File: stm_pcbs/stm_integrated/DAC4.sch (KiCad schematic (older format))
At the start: 21 parts, among them P4 BNC, U10 AD8676, U11 AD5791, U12 AD8675

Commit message: working on Kicad of 3rd Dec
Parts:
- C49, C51, C53, C55, C56, C59, C60, C63, C64: symbol C -> device:C
- C50, C52, C54, C57, C58, C61, C62: symbol CP2 -> device:CP1
- P4: symbol BNC -> device:BNC
- R4: symbol R -> device:R
- U10: symbol AD8676 -> ad5791:AD8676
- U11: symbol AD5791 -> ad5791:AD5791
- U12: symbol AD8675 -> ad5791:AD8675
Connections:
- wire segments 111 -> 126
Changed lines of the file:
@@
-EESchema Schematic File Version 2
-LIBS:power
-LIBS:device
-LIBS:transistors
-LIBS:conn
-LIBS:linear
-LIBS:regul
-LIBS:74xx
-LIBS:cmos4000
-LIBS:adc-dac
-LIBS:memory
-LIBS:xilinx
-LIBS:special
-LIBS:microcontrollers
-LIBS:dsp
-LIBS:microchip
-LIBS:analog_switches
-LIBS:motorola
-LIBS:texas
-LIBS:intel
-LIBS:audio
-LIBS:interface
-LIBS:digital-audio
-LIBS:philips
-LIBS:display
-LIBS:cypress
-LIBS:siliconi
-LIBS:opto
-LIBS:atmel
-LIBS:contrib
-LIBS:valves
-LIBS:ad5791
+EESchema Schematic File Version 4
 LIBS:stmshieldfull-cache
-LIBS:powerbrd-cache
-LIBS:LTC1859-cache
-EELAYER 25 0
+EELAYER 26 0
 EELAYER END
 $Descr A4 11693 8268
@@
 $EndDescr
 $Comp
-L AD5791 U11
+L ad5791:AD5791 U11
 U 1 1 5A26063E
 P 5150 3800
@@
 $EndComp
 $Comp
-L AD8675 U12
+L ad5791:AD8675 U12
 U 1 1 5A260645
 P 6850 3450
@@
 $EndComp
 $Comp
-L AD8676 U10
+L ad5791:AD8676 U10
 U 1 1 5A26064C
 P 5050 1750
@@
 $EndComp
 $Comp
-L AD8676 U10
+L ad5791:AD8676 U10
 U 2 1 5A260653
 P 5100 5500
@@
 $EndComp
 $Comp
-L AD8676 U10
+L ad5791:AD8676 U10
 U 3 1 5A26065A
 P 7800 5600
@@
 $EndComp
 $Comp
-L BNC P4
+L device:BNC P4
 U 1 1 5A260661
 P 7950 3450
@@
 -14V
 $Comp
-L AGND #PWR037
+L power:AGND #PWR037
 U 1 1 5A26066E
 P 7950 3800
@@
 3.3V
 $Comp
-L AGND #PWR038
+L power:AGND #PWR038
 U 1 1 5A260677
 P 4950 4900
@@
 $EndComp
 $Comp
-L DGND #PWR039
+L power:DGND #PWR039
 U 1 1 5A26067D
 P 4700 4900
@@
 $EndComp
 $Comp
-L C C51
+L device:C C51
 U 1 1 5A260683
 P 5950 2200
@@
 $EndComp
 $Comp
-L AGND #PWR040
+L power:AGND #PWR040
 U 1 1 5A26068A
 P 6400 2350
@@
 $EndComp
 $Comp
-L C C53
+L device:C C53
 U 1 1 5A260690
 P 6100 4600
@@
 $EndComp
 $Comp
-L AGND #PWR041
+L power:AGND #PWR041
 U 1 1 5A260697
 P 6500 4750
@@
 $EndComp
 $Comp
-L C C49
+L device:C C49
 U 1 1 5A2606AB
 P 3950 1900
@@
 $EndComp
 $Comp
-L DGND #PWR042
+L power:DGND #PWR042
 U 1 1 5A2606B2
 P 3700 1700
@@
 $EndComp
 $Comp
-L C C56
+L device:C C56
 U 1 1 5A2606B8
 P 7450 5600
@@
 $EndComp
 $Comp
-L C C63
+L device:C C63
 U 1 1 5A2606BF
 P 8850 5450
@@
 $EndComp
 $Comp
-L C C64
+L device:C C64
 U 1 1 5A2606C6
 P 8850 6000
@@
 $EndComp
 $Comp
-L AGND #PWR043
+L power:AGND #PWR043
 U 1 1 5A2606CD
 P 9100 5700
@@
 $EndComp
 $Comp
-L AGND #PWR044
+L power:AGND #PWR044
 U 1 1 5A2606D3
 P 9100 6250
@@
 $EndComp
 $Comp
-L C C55
+L device:C C55
 U 1 1 5A2606D9
 P 7200 5600
@@
 $EndComp
 $Comp
-L CP2 C61
+L device:CP1 C61
 U 1 1 5A2606E0
 P 8600 5450
@@
 $EndComp
 $Comp
-L CP2 C62
+L device:CP1 C62
 U 1 1 5A2606E7
 P 8600 6000
@@
 $EndComp
 $Comp
-L CP2 C54
+L device:CP1 C54
 U 1 1 5A2606EE
 P 6100 4850
@@
 $EndComp
 $Comp
-L CP2 C52
+L device:CP1 C52
 U 1 1 5A2606F5
 P 5950 2450
@@
 $EndComp
 $Comp
-L CP2 C50
+L device:CP1 C50
 U 1 1 5A2606FC
 P 4200 1900
@@
 RESET4
 $Comp
-L CP2 C57
+L device:CP1 C57
 U 1 1 5A26070A
 P 7500 3100
@@
 $EndComp
 $Comp
-L CP2 C58
+L device:CP1 C58
 U 1 1 5A260711
 P 7500 3850
@@
 $EndComp
 $Comp
-L C C59
+L device:C C59
 U 1 1 5A260718
 P 7700 3100
@@
 $EndComp
 $Comp
-L C C60
+L device:C C60
 U 1 1 5A26071F
 P 7700 3850
@@
 $EndComp
 $Comp
-L AGND #PWR045
+L power:AGND #PWR045
 U 1 1 5A260726
 P 7400 3300
@@
 $EndComp
 $Comp
-L AGND #PWR046
+L power:AGND #PWR046
 U 1 1 5A26072C
 P 7500 4150
@@
 	6000 3350 6550 3350
 Wire Wire Line
-	7150 3450 7800 3450
+	7150 3450 7250 3450
 Wire Wire Line
 	5000 1350 5000 1500
@@
 	5000 5750 5000 5900
 Wire Wire Line
-	7350 5250 7900 5250
-Wire Wire Line
-	7350 5950 7900 5950
+	7350 5250 7700 5250
 Wire Wire Line
 	6550 3550 6000 3550
@@
 Connection ~ 7250 3450
 Wire Wire Line
-	6850 3100 7050 3100
-Wire Wire Line
-	6850 3800 7000 3800
+	6850 3100 6950 3100
+Wire Wire Line
+	6850 3800 6950 3800
 Wire Wire Line
 	7950 3650 7950 3800
 Wire Wire Line
-	5700 2050 5700 2350
+	5700 2050 5700 2200
 Wire Wire Line
 	5400 4700 5400 4850
@@
 	4900 2400 4900 2600
 Wire Wire Line
-	4350 2400 4900 2400
+	4350 2400 4550 2400
 Wire Wire Line
 	4750 2400 4750 2600
@@
 Connection ~ 5700 2300
 Wire Wire Line
-	6150 2200 6150 2450
+	6150 2200 6150 2300
 Wire Wire Line
 	6150 2300 6400 2300
@@
 	5400 4700 5900 4700
 Wire Wire Line
-	5900 4600 5900 4850
-Wire Wire Line
-	6300 4600 6300 4850
+	5900 4600 5900 4700
+Wire Wire Line
+	6300 4600 6300 4700
 Connection ~ 5900 4700
 Wire Wire Line
@@
 Connection ~ 6300 4700
 Wire Wire Line
-	3950 1700 4200 1700
-Wire Wire Line
-	3950 2100 4200 2100
-Wire Wire Line
-	4050 2100 4550 2100
+	3950 1700 4050 1700
 Wire Wire Line
 	4550 2100 4550 2400
 Connection ~ 4550 2400
-Connection ~ 4050 2100
 Wire Wire Line
 	4050 1700 4050 1450
@@
 Connection ~ 4050 1700
 Wire Wire Line
-	8600 5250 8850 5250
+	8600 5250 8700 5250
 Wire Wire Line
 	8600 5650 8850 5650
 Wire Wire Line
-	7850 5800 8850 5800
-Wire Wire Line
 	8600 6200 8850 6200
 Wire Wire Line
-	7200 5400 7450 5400
-Wire Wire Line
-	7200 5800 7450 5800
+	7200 5400 7350 5400
+Wire Wire Line
+	7200 5800 7350 5800
 Wire Wire Line
 	7350 5400 7350 5250
@@
 Wire Wire Line
 	7350 5800 7350 5950
-Connection ~ 7700 5950
 Connection ~ 7350 5800
 Wire Wire Line
-	7700 5950 7850 5950
-Wire Wire Line
 	7850 5950 7850 5800
-Connection ~ 8600 5800
 Wire Wire Line
 	7700 5250 7700 5150
@@
 	8850 5700 9100 5700
 Wire Wire Line
-	8850 5600 8850 5700
+	8850 5600 8850 5650
 Wire Wire Line
 	8850 6250 9100 6250
 Wire Wire Line
-	8850 6150 8850 6250
+	8850 6150 8850 6200
 Wire Wire Line
 	3300 4100 3950 4100
@@
 Connection ~ 7800 5950
 Wire Wire Line
-	7500 2900 7700 2900
-Wire Wire Line
-	7400 3300 7700 3300
-Wire Wire Line
-	7500 3650 7700 3650
-Wire Wire Line
 	7500 4050 7700 4050
-Wire Wire Line
-	7600 2900 6950 2900
 Wire Wire Line
 	6950 2900 6950 3100
 Connection ~ 6950 3100
-Connection ~ 7600 2900
-Wire Wire Line
-	7600 3650 6950 3650
 Wire Wire Line
 	6950 3650 6950 3800
 Connection ~ 6950 3800
-Connection ~ 7600 3650
-Connection ~ 7500 4050
-Connection ~ 7500 3300
-$Comp
-L R R4
+$Comp
+L device:R R4
 U 1 1 5A2607A6
 P 7250 4550
@@
 $EndComp
 $Comp
-L AGND #PWR047
+L power:AGND #PWR047
 U 1 1 5A2607AD
 P 7000 4650
@@
 $EndComp
 $Comp
-L DGND #PWR048
+L power:DGND #PWR048
 U 1 1 5A2607B3
 P 7500 4650
@@
 Wire Wire Line
 	8850 5250 8850 5300
+Wire Wire Line
+	7250 3450 7800 3450
+Wire Wire Line
+	4750 2400 4900 2400
+Wire Wire Line
+	5700 2200 5700 2300
+Wire Wire Line
+	5700 2300 5700 2350
+Wire Wire Line
+	6150 2300 6150 2450
+Wire Wire Line
+	5900 4700 5900 4850
+Wire Wire Line
+	6300 4700 6300 4850
+Wire Wire Line
+	4550 2400 4750 2400
+Wire Wire Line
+	4050 1700 4200 1700
+Wire Wire Line
+	7700 5250 7800 5250
+Wire Wire Line
+	7350 5400 7450 5400
+Wire Wire Line
+	7350 5800 7450 5800
+Wire Wire Line
+	8700 5250 8850 5250
+Wire Wire Line
+	7800 5250 7900 5250
+Wire Wire Line
+	6950 3100 7050 3100
+Wire Wire Line
+	6950 3800 7000 3800
+Wire Wire Line
+	8850 6200 8850 6250
+Wire Wire Line
+	8850 5650 8850 5700
+Wire Wire Line
+	7850 5800 8850 5800
+Wire Wire Line
+	7400 3300 7700 3300
+Wire Wire Line
+	3950 2100 4550 2100
+Wire Wire Line
+	7350 5950 7800 5950
+Wire Wire Line
+	7800 5950 7900 5950
+Wire Wire Line
+	6950 2900 7700 2900
+Wire Wire Line
+	6950 3650 7700 3650
 $EndSCHEMATC

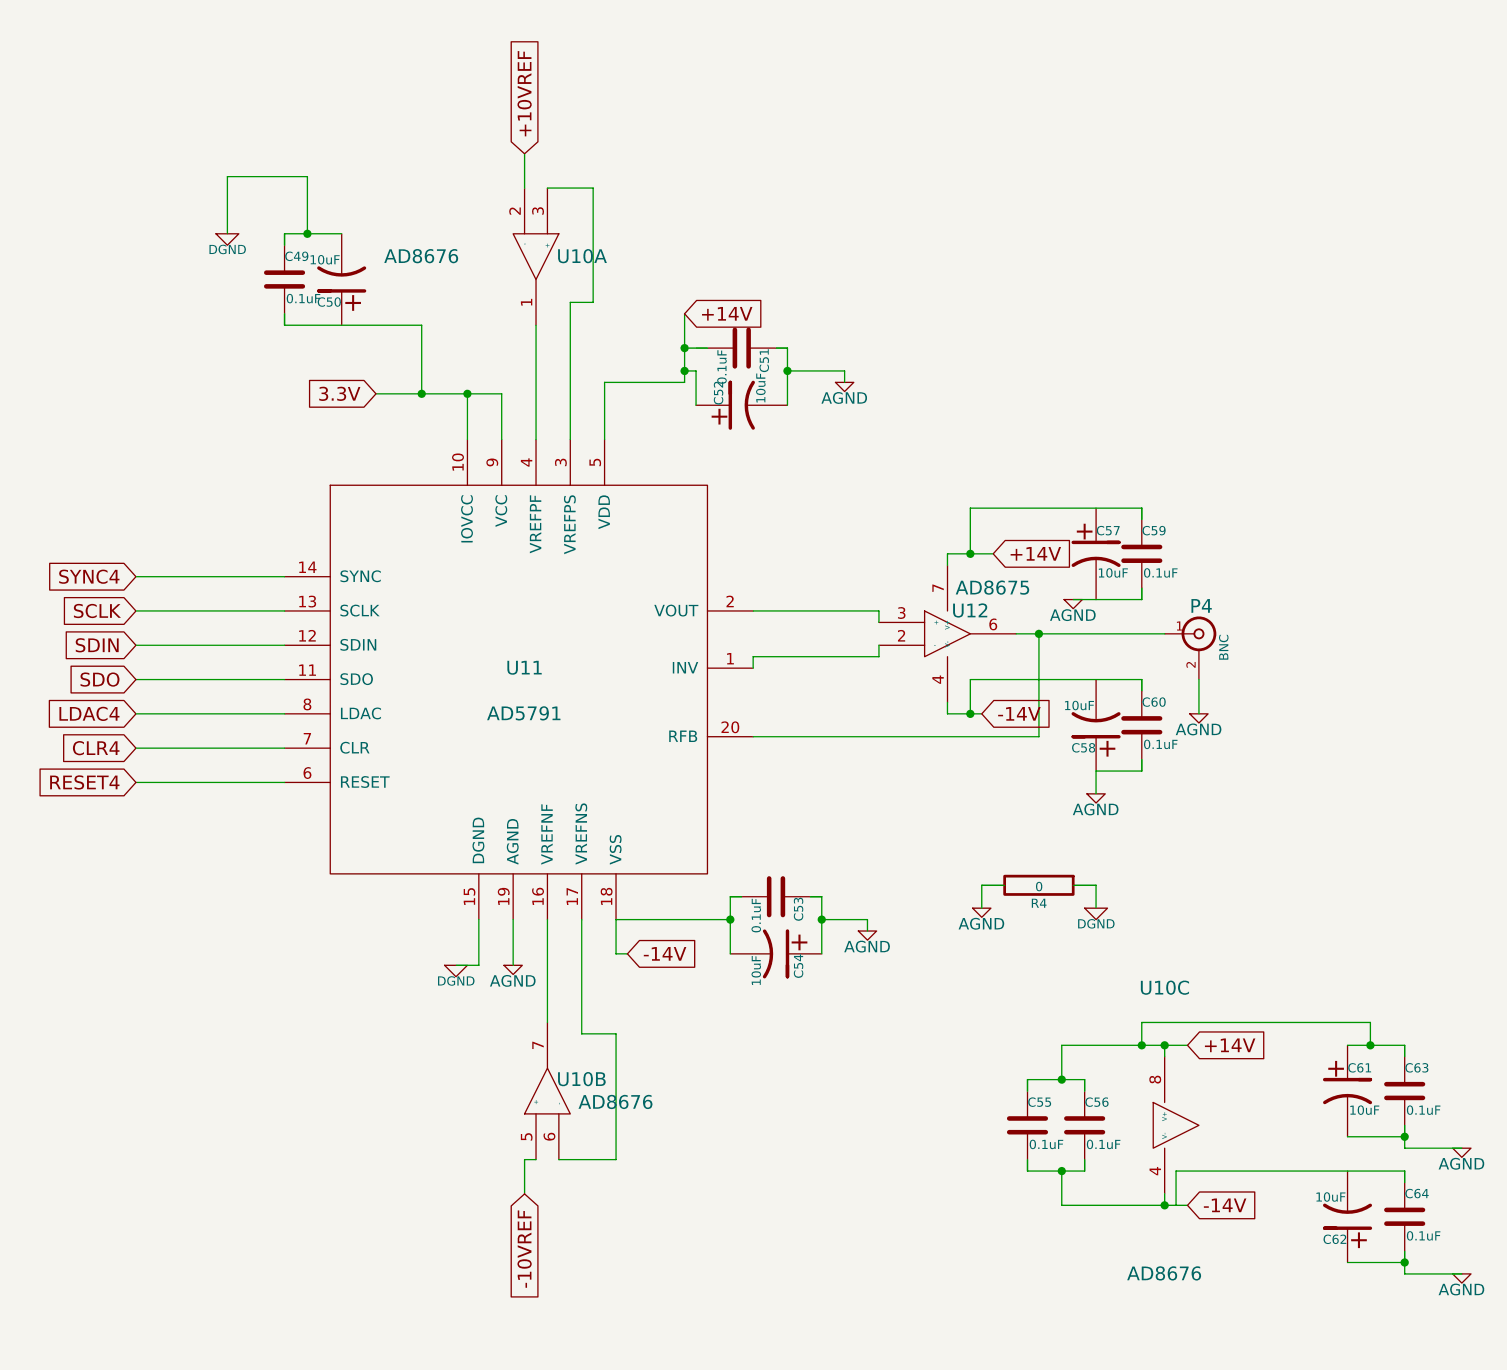
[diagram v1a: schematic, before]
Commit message: fixing more borkage
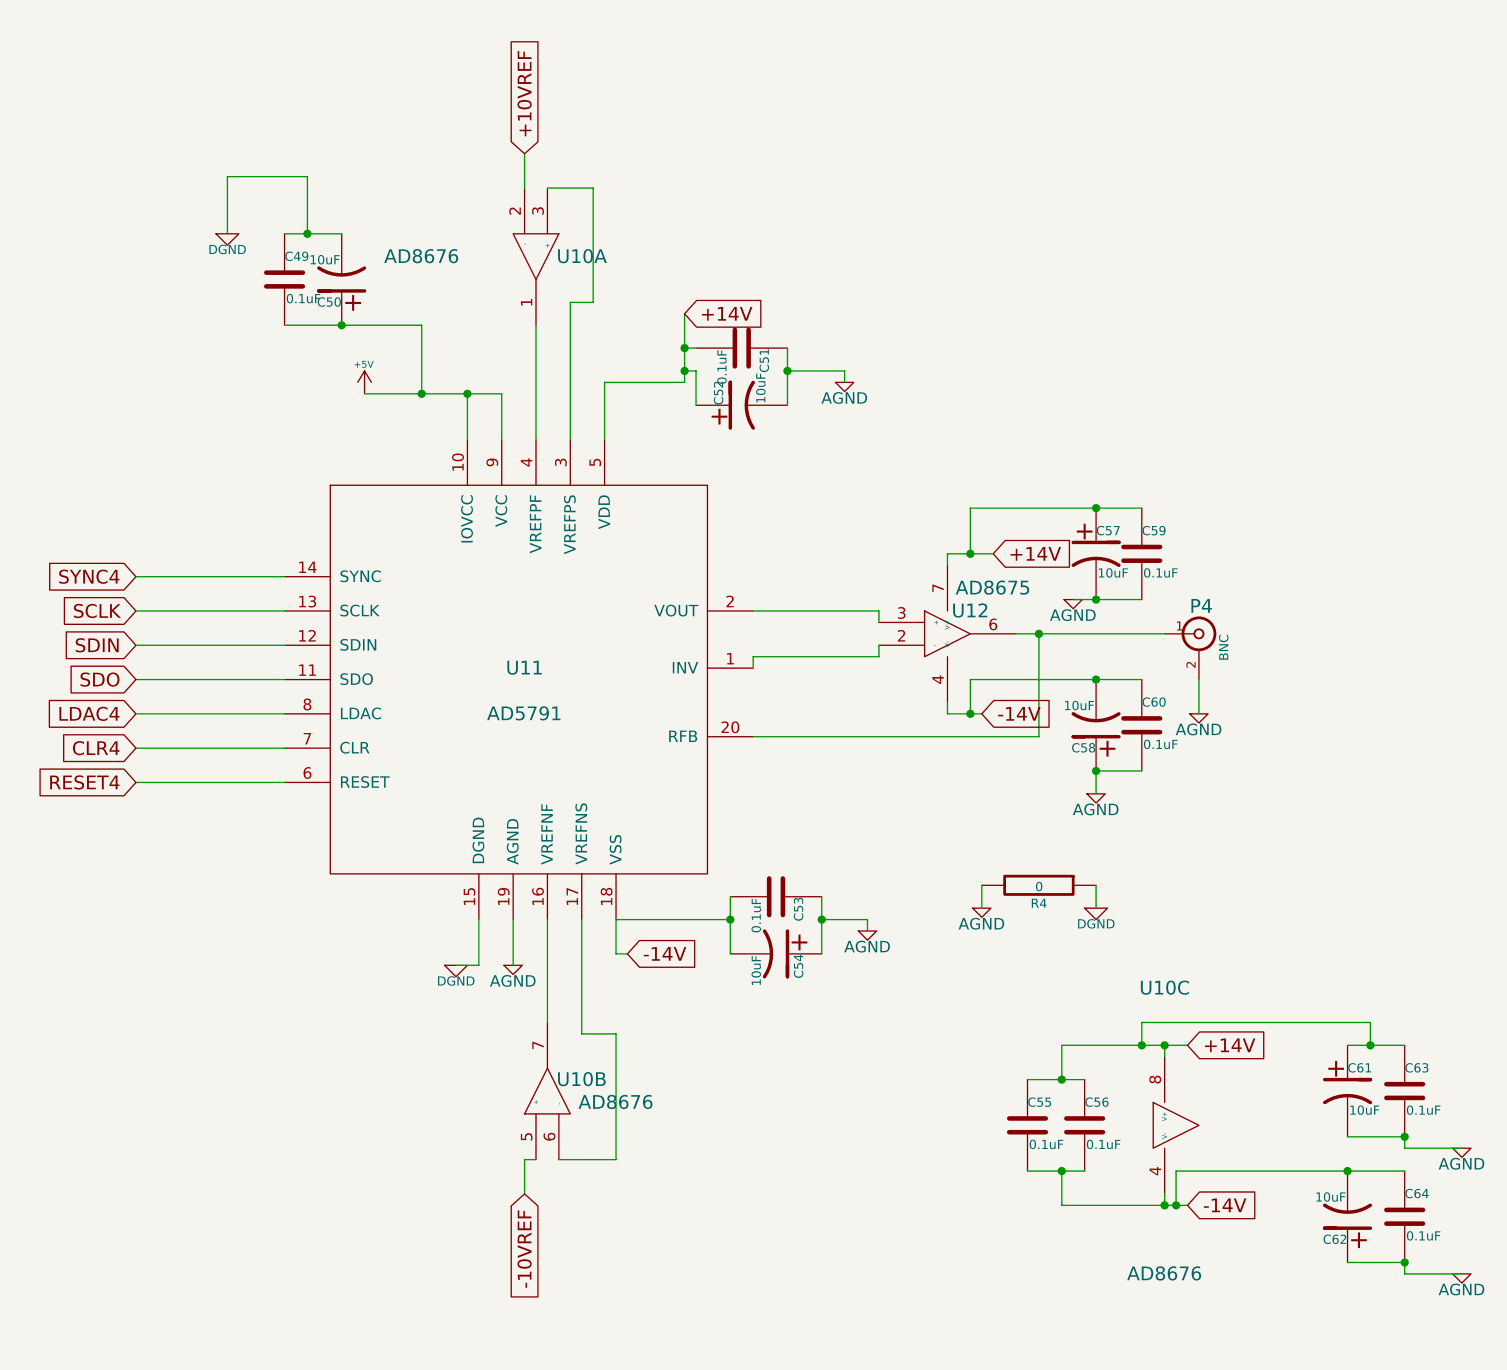
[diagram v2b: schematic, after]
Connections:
- net labels added: +5V
- net labels removed: 3.3V
- wire segments 126 -> 113
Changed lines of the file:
@@
 Text GLabel 5450 4850 2    60   Input ~ 0
 -14V
-Text GLabel 4350 2400 0    60   Input ~ 0
-3.3V
 $Comp
 L power:AGND #PWR038
@@
 	7950 3650 7950 3800
 Wire Wire Line
-	5700 2050 5700 2200
-Wire Wire Line
 	5400 4700 5400 4850
 Wire Wire Line
@@
 Wire Wire Line
 	4900 2400 4900 2600
-Wire Wire Line
-	4350 2400 4550 2400
 Wire Wire Line
 	4750 2400 4750 2600
@@
 Wire Wire Line
 	5350 2350 5350 2600
-Wire Wire Line
-	5700 2200 5800 2200
-Connection ~ 5700 2200
 Wire Wire Line
 	5750 2450 5750 2300
@@
 Connection ~ 7350 5800
 Wire Wire Line
-	7850 5950 7850 5800
-Wire Wire Line
 	7700 5250 7700 5150
 Wire Wire Line
@@
 	8850 5700 9100 5700
 Wire Wire Line
-	8850 5600 8850 5650
-Wire Wire Line
 	8850 6250 9100 6250
-Wire Wire Line
-	8850 6150 8850 6200
 Wire Wire Line
 	3300 4100 3950 4100
@@
 	7000 4550 7000 4650
 Wire Wire Line
-	7700 3650 7700 3700
-Wire Wire Line
-	7700 4050 7700 4000
-Wire Wire Line
-	7500 4550 7400 4550
-Wire Wire Line
-	7100 4550 7000 4550
-Wire Wire Line
-	6250 4600 6300 4600
-Wire Wire Line
-	5950 4600 5900 4600
-Wire Wire Line
-	7700 2900 7700 2950
-Wire Wire Line
-	7700 3300 7700 3250
-Wire Wire Line
-	3950 2050 3950 2100
-Wire Wire Line
-	3950 1750 3950 1700
-Wire Wire Line
-	6100 2200 6150 2200
-Wire Wire Line
 	3300 3200 3950 3200
 Wire Wire Line
 	7500 4150 7500 4050
-Wire Wire Line
-	7450 5400 7450 5450
-Wire Wire Line
-	7450 5800 7450 5750
-Wire Wire Line
-	7200 5800 7200 5750
-Wire Wire Line
-	7200 5450 7200 5400
-Wire Wire Line
-	8850 5800 8850 5850
 Connection ~ 8850 6200
 Connection ~ 8850 5650
 Wire Wire Line
-	8850 5250 8850 5300
-Wire Wire Line
 	7250 3450 7800 3450
 Wire Wire Line
 	4750 2400 4900 2400
 Wire Wire Line
+	5700 2300 5700 2350
+Wire Wire Line
+	6150 2300 6150 2450
+Wire Wire Line
+	5900 4700 5900 4850
+Wire Wire Line
+	6300 4700 6300 4850
+Wire Wire Line
+	4550 2400 4750 2400
+Wire Wire Line
+	4050 1700 4200 1700
+Wire Wire Line
+	7700 5250 7800 5250
+Wire Wire Line
+	7350 5400 7450 5400
+Wire Wire Line
+	7350 5800 7450 5800
+Wire Wire Line
+	8700 5250 8850 5250
+Wire Wire Line
+	7800 5250 7900 5250
+Wire Wire Line
+	6950 3100 7050 3100
+Wire Wire Line
+	6950 3800 7000 3800
+Wire Wire Line
+	8850 6200 8850 6250
+Wire Wire Line
+	8850 5650 8850 5700
+Wire Wire Line
+	7850 5800 8600 5800
+Wire Wire Line
+	7400 3300 7500 3300
+Wire Wire Line
+	3950 2100 4200 2100
+Wire Wire Line
+	7350 5950 7800 5950
+Wire Wire Line
+	7800 5950 7850 5950
+Wire Wire Line
+	6950 2900 7500 2900
+Wire Wire Line
+	6950 3650 7500 3650
+$Comp
+L power:+5V #PWR?
+U 1 1 5A4F308A
+P 4300 2400
+F 0 "#PWR?" H 4300 2490 20  0001 C CNN
+F 1 "+5V" H 4296 2528 30  0000 C CNN
+F 2 "" H 4300 2400 60  0001 C CNN
+F 3 "" H 4300 2400 60  0001 C CNN
+	1    4300 2400
+	1    0    0    -1
+$EndComp
+Wire Wire Line
+	4300 2400 4550 2400
+Connection ~ 7500 3650
+Wire Wire Line
+	7500 3650 7700 3650
+Connection ~ 7500 4050
+Connection ~ 7500 2900
+Wire Wire Line
+	7500 2900 7700 2900
+Connection ~ 7500 3300
+Wire Wire Line
+	7500 3300 7700 3300
+Wire Wire Line
+	7850 5800 7850 5950
+Connection ~ 7850 5950
+Wire Wire Line
+	7850 5950 7900 5950
+Connection ~ 8600 5800
+Wire Wire Line
+	8600 5800 8850 5800
+Connection ~ 4200 2100
+Wire Wire Line
+	4200 2100 4550 2100
+Wire Wire Line
+	5700 2050 5700 2200
+Wire Wire Line
+	5750 2200 5700 2200
+Connection ~ 5700 2200
+Wire Wire Line
 	5700 2200 5700 2300
-Wire Wire Line
-	5700 2300 5700 2350
-Wire Wire Line
-	6150 2300 6150 2450
-Wire Wire Line
-	5900 4700 5900 4850
-Wire Wire Line
-	6300 4700 6300 4850
-Wire Wire Line
-	4550 2400 4750 2400
-Wire Wire Line
-	4050 1700 4200 1700
-Wire Wire Line
-	7700 5250 7800 5250
-Wire Wire Line
-	7350 5400 7450 5400
-Wire Wire Line
-	7350 5800 7450 5800
-Wire Wire Line
-	8700 5250 8850 5250
-Wire Wire Line
-	7800 5250 7900 5250
-Wire Wire Line
-	6950 3100 7050 3100
-Wire Wire Line
-	6950 3800 7000 3800
-Wire Wire Line
-	8850 6200 8850 6250
-Wire Wire Line
-	8850 5650 8850 5700
-Wire Wire Line
-	7850 5800 8850 5800
-Wire Wire Line
-	7400 3300 7700 3300
-Wire Wire Line
-	3950 2100 4550 2100
-Wire Wire Line
-	7350 5950 7800 5950
-Wire Wire Line
-	7800 5950 7900 5950
-Wire Wire Line
-	6950 2900 7700 2900
-Wire Wire Line
-	6950 3650 7700 3650
 $EndSCHEMATC
